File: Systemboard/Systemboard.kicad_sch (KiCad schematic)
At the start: 17 parts, among them J1 Conn_01x60, J108 Prog BT, U103 ESP32-WROOM-32U

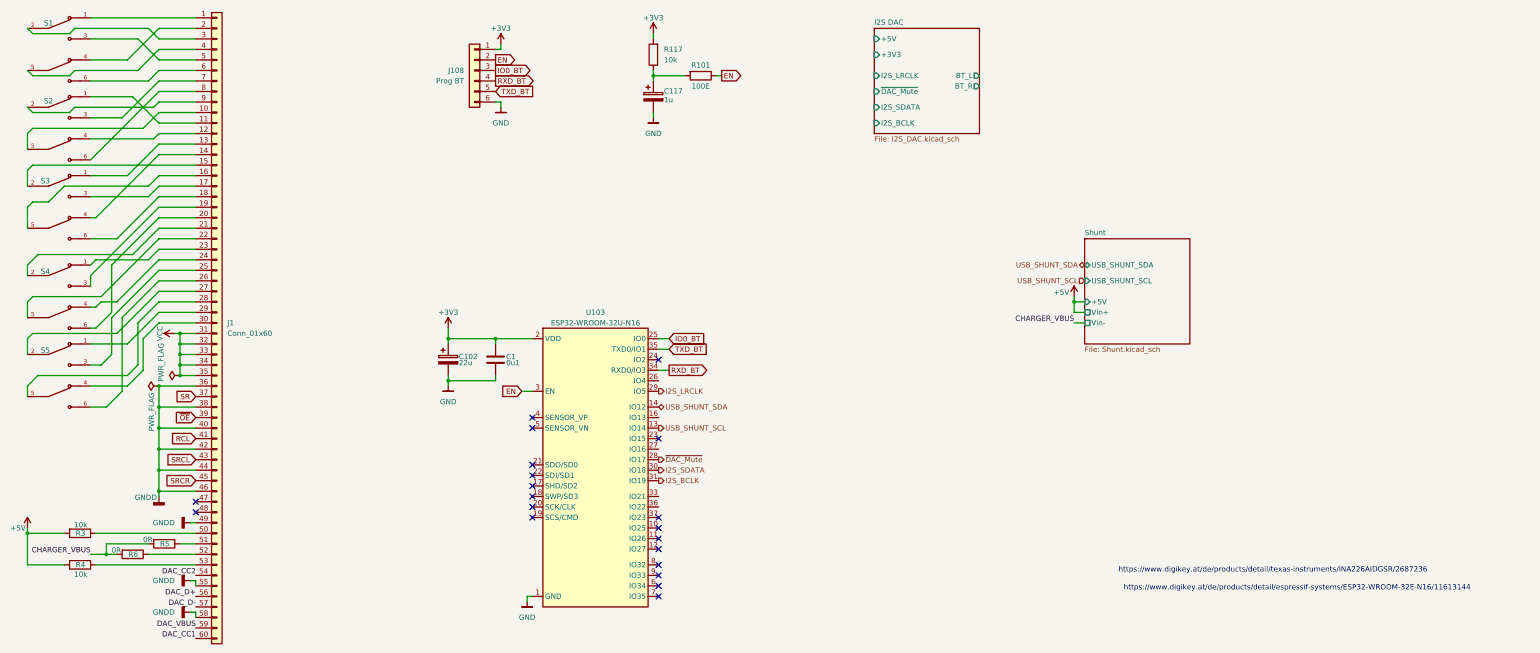
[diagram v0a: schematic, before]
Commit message: user save
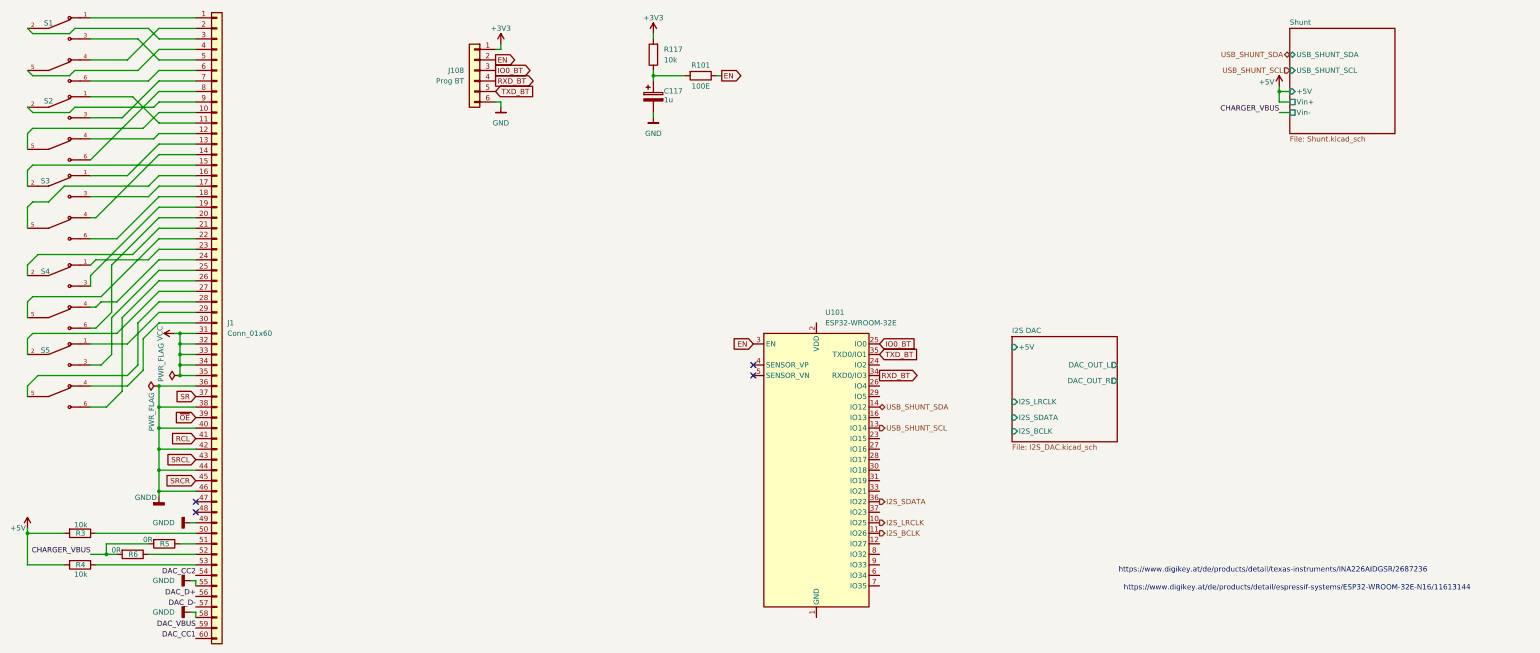
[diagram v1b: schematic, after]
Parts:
- removed C1: 0u1, Capacitor_THT:C_Disc_D4.7mm_W2.5mm_P5.00mm, symbol Device:C
- removed C102: 22u, Capacitor_THT:CP_Radial_D5.0mm_P2.00mm, symbol Device:C_Polarized
- removed U103: ESP32-WROOM-32U, RF_Module:ESP32-WROOM-32U, symbol modules:ESP32-WROOM-32U-N16
- added U101: ESP32-WROOM-32E, RF_Module:ESP32-WROOM-32D, symbol RF_Module:ESP32-WROOM-32E
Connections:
- net EN: now also U101.3 (EN)
- net I2S_BCLK: now also U101.11 (IO26)
- net I2S_LRCLK: now also U101.10 (IO25)
- net I2S_SDATA: now also U101.36 (IO22)
- net IO0_BT: now also U101.25 (IO0)
- net RXD_BT: now also U101.34 (RXD0/IO3)
- net TXD_BT: now also U101.35 (TXD0/IO1)
- net USB_SHUNT_SCL: now also U101.13 (IO14)
- net USB_SHUNT_SDA: now also U101.14 (IO12)
- new net: U101.1 (GND), U101.15 (GND), U101.38 (GND), U101.39 (GND)
- no-connect marks 20 -> 4
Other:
- sheet I2S DAC ports: added DAC_OUT_L, DAC_OUT_R; removed +3V3, BT_L, BT_R, ~{DAC_Mute}
